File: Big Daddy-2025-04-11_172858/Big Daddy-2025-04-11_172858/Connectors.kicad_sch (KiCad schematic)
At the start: 7 parts, among them J10 Conn_01x02, J11 Conn_01x23, J12 Conn_01x14, J13 Conn_01x14, J15 Conn_01x02, J17 Conn_01x14, J8 Conn_01x14

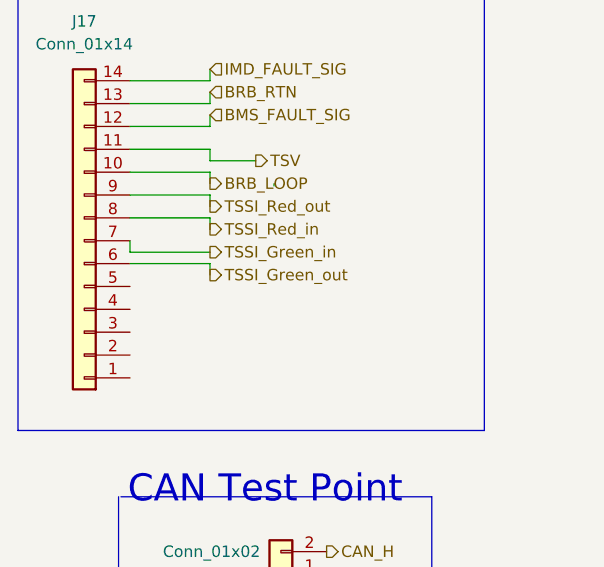
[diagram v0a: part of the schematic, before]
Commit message: Rerouted PCB
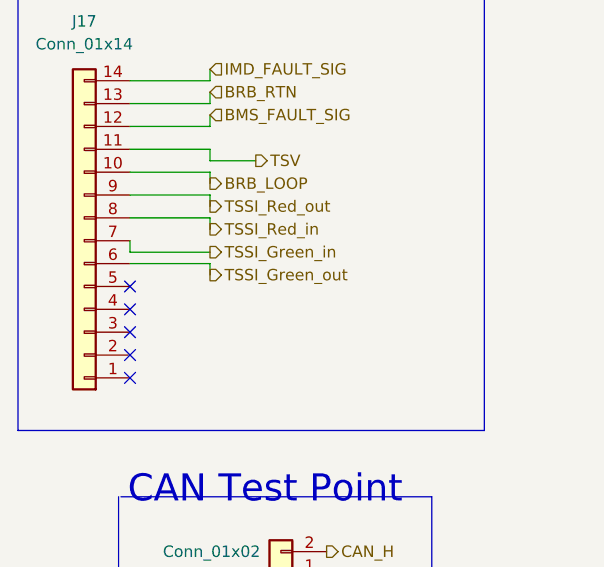
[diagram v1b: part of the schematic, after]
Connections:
- no-connect marks 0 -> 5
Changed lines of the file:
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@@
 		(color 0 0 0 0)
+	)
+	(no_connect
+		(at 30.48 140.97)
+	)
+	(no_connect
+		(at 30.48 133.35)
+	)
+	(no_connect
+		(at 30.48 143.51)
+	)
+	(no_connect
+		(at 30.48 138.43)
+	)
+	(no_connect
+		(at 30.48 135.89)
 	)
 	(polyline
@@
 		)
 		(stroke
-			(width 0)
-			(type default)
-		)
-	)
-	(wire
-		(pts
-			(xy 46.482 122.174) (xy 46.482 121.92)
-		)
-		(stroke
